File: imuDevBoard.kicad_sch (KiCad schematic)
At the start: 22 parts, among them J1 USB_C_Receptacle_USB2.0_16P, SW1 SW_Push, SW2 SW_SPDT, U1 RP2350A, U2 W25Q128JVS, U3 TLV75533PDBV, Y1 Crystal_GND24

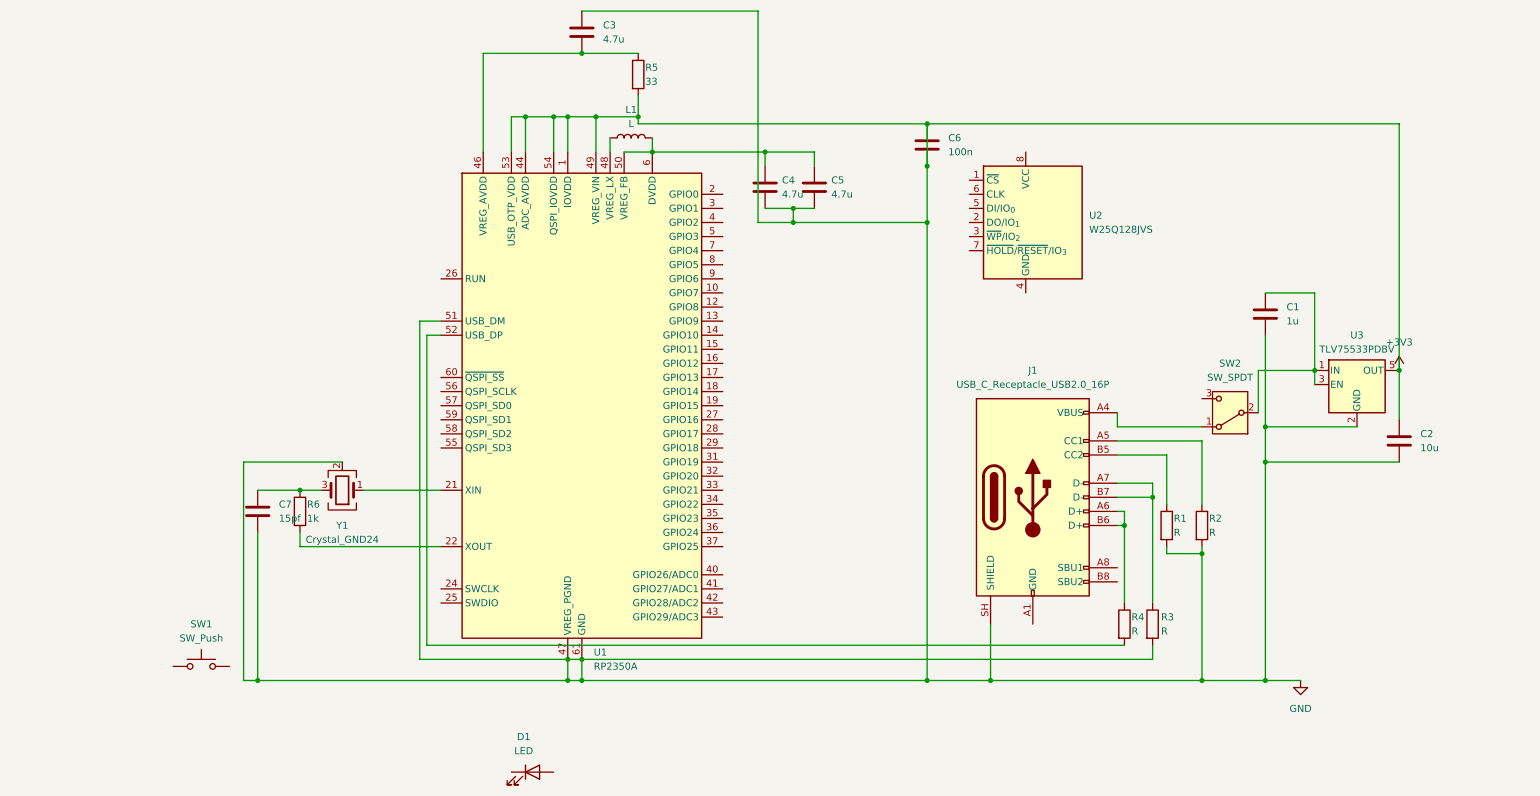
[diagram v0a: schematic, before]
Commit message: everything but imu pretty much done
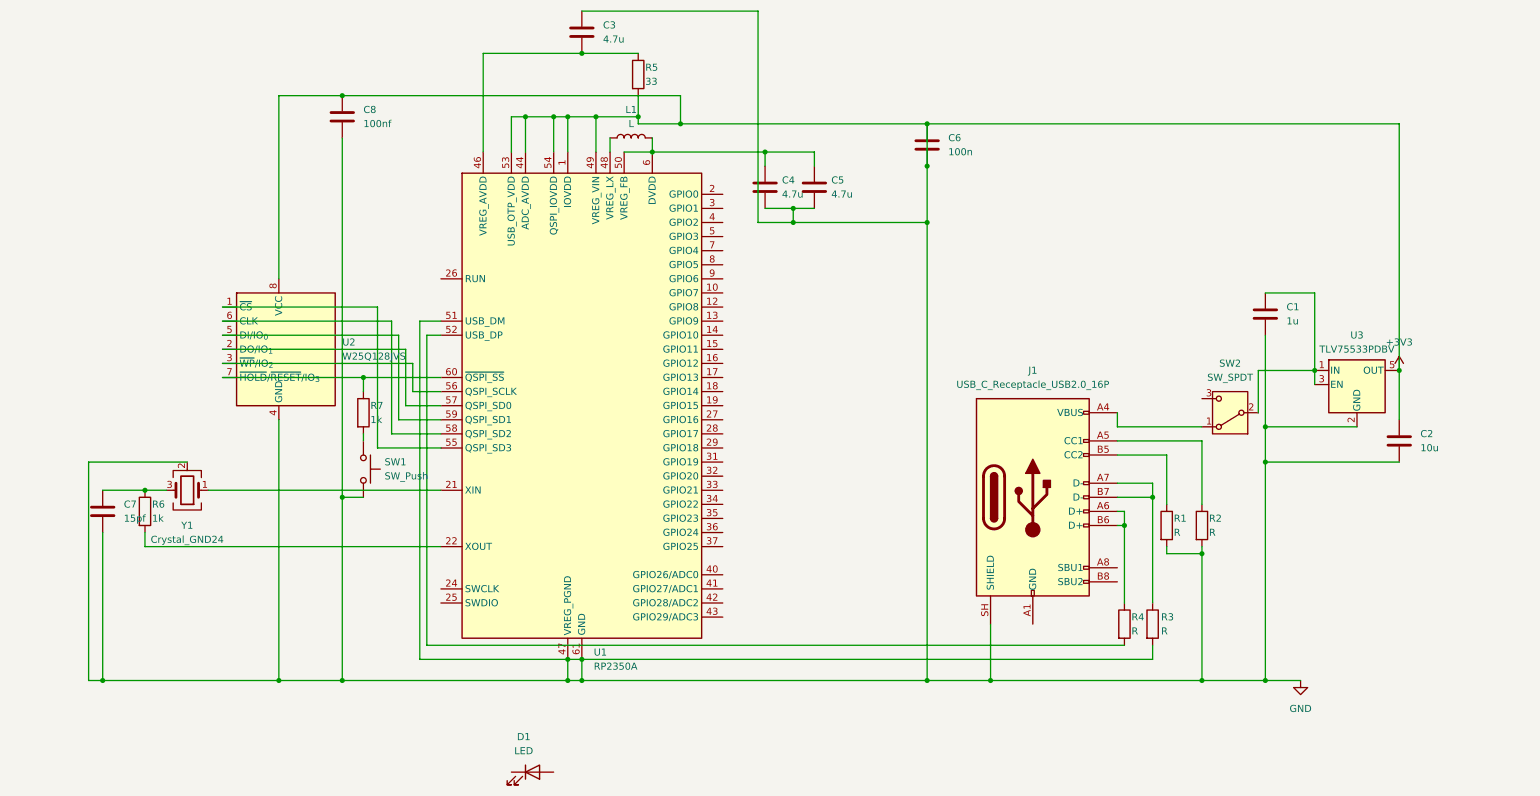
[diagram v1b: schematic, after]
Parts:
- added C8: 100nf, symbol Device:C
- added R7: 1k, symbol Device:R
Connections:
- net +3V3: now also SW1.2, U2.4 (GND), U2.8 (VCC), C8.1, C8.2
- net at SW1.1: now also R7.2
- net at U1.55 (QSPI_SD3): now also U2.1 (~{CS})
- net at U1.56 (QSPI_SCLK): now also U2.3 (~{WP}/IO_{2})
- net at U1.57 (QSPI_SD0): now also U2.2 (DO/IO_{1})
- net at U1.58 (QSPI_SD2): now also U2.6 (CLK)
- net at U1.59 (QSPI_SD1): now also U2.5 (DI/IO_{0})
- net at U1.60 (~{QSPI_SS}): now also U2.7 (~{HOLD}/~{RESET}/IO_{3}), R7.1
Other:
- moved on the sheet: C7, R6, U2, Y1

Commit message: finish sch
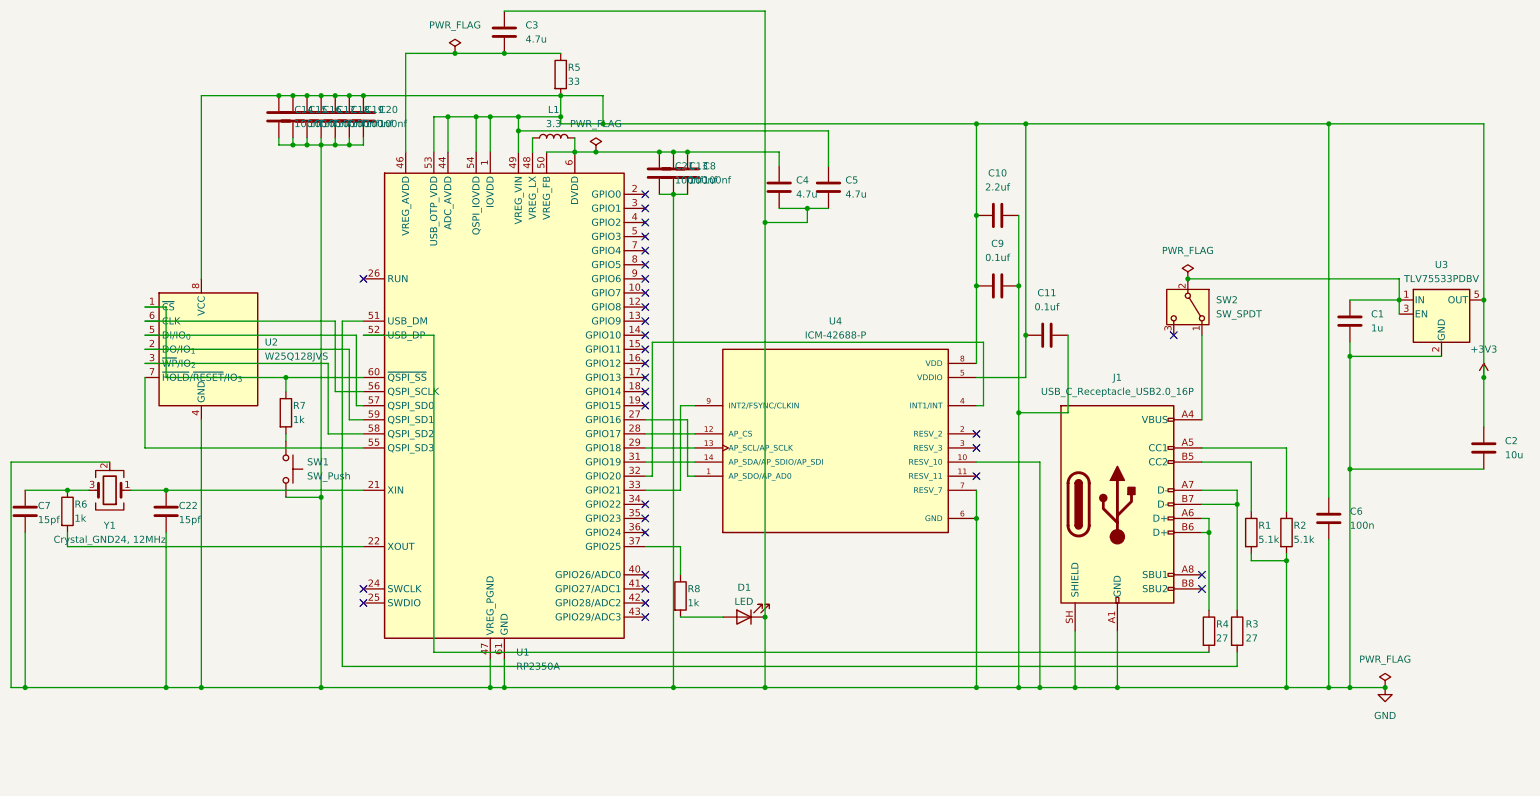
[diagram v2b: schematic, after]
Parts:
- added C10: 2.2uf, Capacitor_SMD:C_0402_1005Metric, symbol Device:C
- added C11, C9: 0.1uf, Capacitor_SMD:C_0402_1005Metric, symbol Device:C
- added C13, C14, C15, C16, C17, C18, C19, C20, C21: 100nf, Capacitor_SMD:C_0402_1005Metric, symbol Device:C
- added C22: 15pf, Capacitor_SMD:C_0402_1005Metric, symbol Device:C
- added R8: 1k, Resistor_SMD:R_0402_1005Metric, symbol Device:R
- added U4: ICM-42688-P, kicad-includes:ICM-42688-P, symbol ICM-42688-P:ICM-42688-P
- C1, C3, C4, C5, C6, C7, C8: footprint (none) -> Capacitor_SMD:C_0402_1005Metric
- C2: footprint (none) -> Capacitor_SMD:C_0603_1608Metric
- D1: footprint (none) -> LED_SMD:LED_0603_1608Metric
- J1: footprint (none) -> Connector_USB:USB_C_Receptacle_HRO_TYPE-C-31-M-12
- L1: value L -> 3.3; footprint (none) -> kicad-includes:AOTA-B2016
- R1, R2: value R -> 5.1k; footprint (none) -> Resistor_SMD:R_0402_1005Metric
- R3, R4: value R -> 27; footprint (none) -> Resistor_SMD:R_0402_1005Metric
- R5, R6, R7: footprint (none) -> Resistor_SMD:R_0402_1005Metric
- SW1: footprint (none) -> Button_Switch_SMD:SW_Push_1P1T_NO_Vertical_Wuerth_434133025816
- SW2: footprint (none) -> Button_Switch_SMD:SW_SPDT_Shouhan_MSK12C02
- Y1: value Crystal_GND24 -> Crystal_GND24, 12MHz; footprint (none) -> Crystal:Crystal_SMD_3225-4Pin_3.2x2.5mm
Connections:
- net +3V3: now also C5.2, C10.1, C11.1, C14.2, C15.2, C16.2, C17.2, C18.2, C19.2, C20.2, C9.1, U4.5 (VDDIO), U4.8 (VDD); no longer C1.2, C2.2, C3.1, C4.1, C5.1, C6.1, C7.1, C8.1, C8.2, J1.SH (SHIELD), R1.2, R2.2, R3.2, SW1.2, U1.47 (VREG_PGND), U1.51 (USB_DM), U1.61 (GND), U2.4 (GND), U3.2 (GND), Y1.2 (G), Y1.4 (G)
- net GND: now reaches D1.1 (K)
- net GND: now also C1.2, C2.2, C3.1, C4.1, C5.1, C6.1, C7.1, C8.1, J1.A1 (GND), J1.A12 (GND), J1.B1 (GND), J1.B12 (GND), J1.SH (SHIELD), R1.2, R2.2, SW1.2, U1.47 (VREG_PGND), U1.61 (GND), U2.4 (GND), U3.2 (GND), Y1.2 (G), Y1.4 (G), C10.2, C11.2, C13.1, C14.1, C15.1, C16.1, C17.1, C18.1, C19.1, C20.1, C21.1, C22.1, C9.2, U4.10 (RESV_10), U4.6 (GND), U4.7 (RESV_7)
- net at D1.2 (A): now also R8.2
- net at U1.21 (XIN), Y1.1: now also C22.2
- net at C4.2, L1.2, U1.23 (DVDD)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: now also C8.2, C13.2, C21.2; no longer C5.2
- net at U1.27 (GPIO16): now also U4.1 (AP_SDO/AP_AD0)
- net at U1.28 (GPIO17): now also U4.12 (AP_CS)
- net at U1.29 (GPIO18): now also U4.13 (AP_SCL/AP_SCLK)
- net at U1.31 (GPIO19): now also U4.14 (AP_SDA/AP_SDIO/AP_SDI)
- net at U1.32 (GPIO20): now also U4.4 (INT1/INT)
- net at U1.33 (GPIO21): now also U4.9 (INT2/FSYNC/CLKIN)
- net at U1.37 (GPIO25): now also R8.1
- net at U1.55 (QSPI_SD3): now also U2.7 (~{HOLD}/~{RESET}/IO_{3}); no longer U2.1 (~{CS})
- net at U1.56 (QSPI_SCLK): now also U2.6 (CLK); no longer U2.3 (~{WP}/IO_{2})
- net at U1.57 (QSPI_SD0): now also U2.5 (DI/IO_{0}); no longer U2.2 (DO/IO_{1})
- net at U1.58 (QSPI_SD2): now also U2.3 (~{WP}/IO_{2}); no longer U2.6 (CLK)
- net at U1.59 (QSPI_SD1): now also U2.2 (DO/IO_{1}); no longer U2.5 (DI/IO_{0})
- net at R7.1, U1.60 (~{QSPI_SS}): now also U2.1 (~{CS}); no longer U2.7 (~{HOLD}/~{RESET}/IO_{3})
- new net: R3.2, U1.51 (USB_DM)
- no-connect marks 0 -> 32
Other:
- moved on the sheet: C1, C2, C3, C4, C5, C6, C7, D1, J1, L1, R1, R2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
